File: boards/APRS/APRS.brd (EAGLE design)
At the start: 50.8 x 38.1 mm, 15 parts

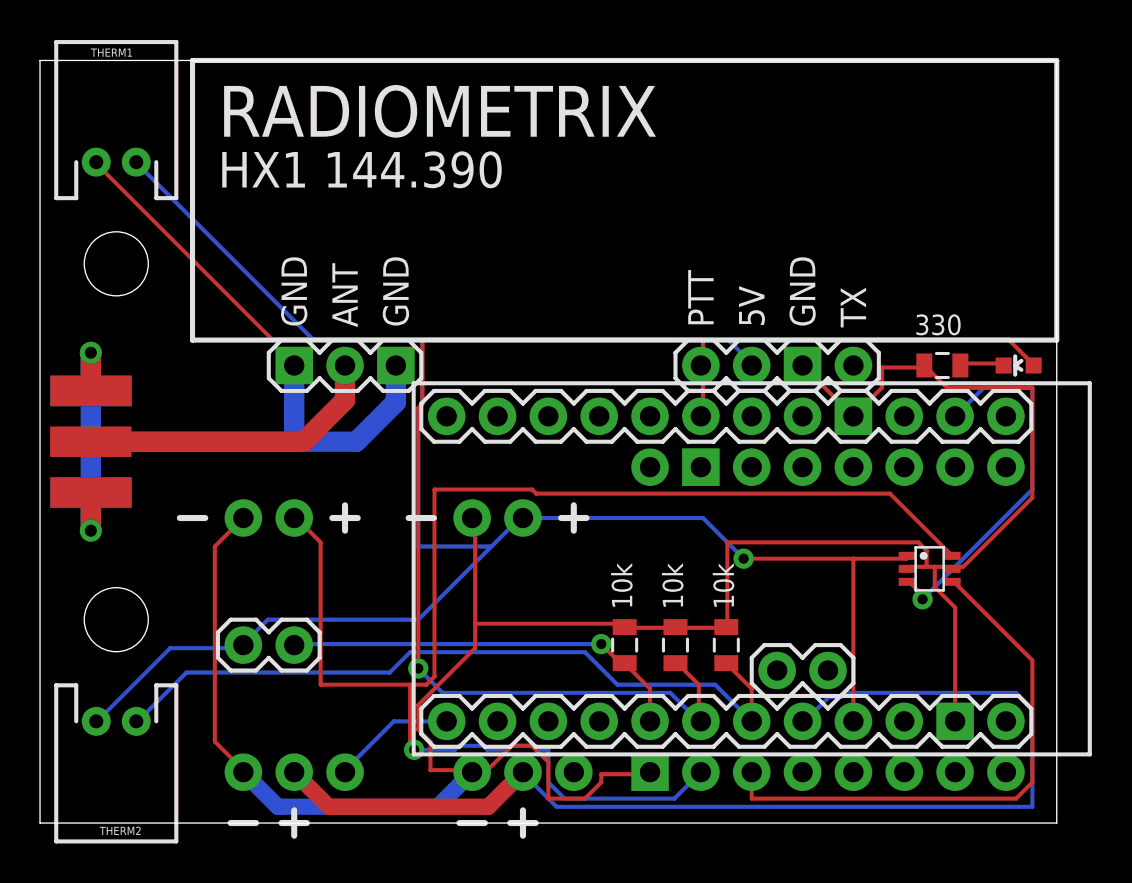
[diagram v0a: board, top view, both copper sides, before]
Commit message: New APRS board, close to ready
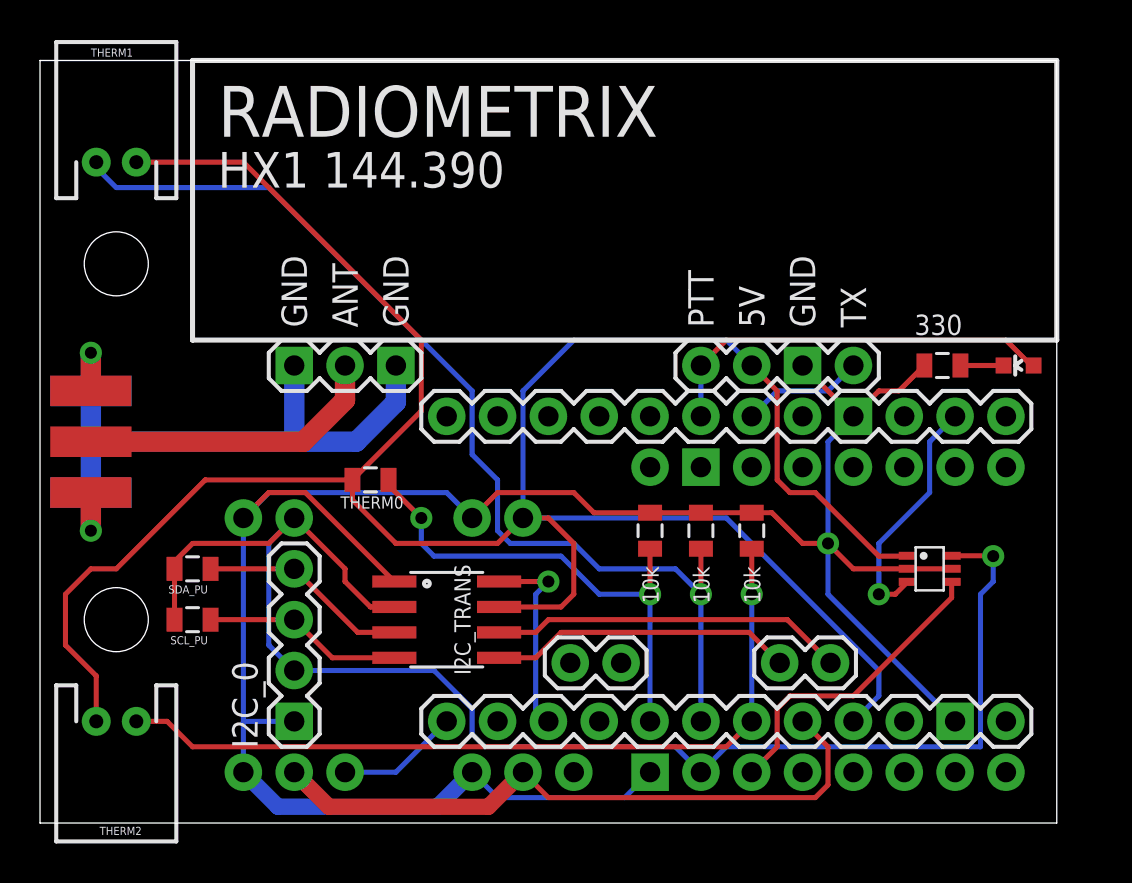
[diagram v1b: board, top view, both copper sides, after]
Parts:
- added I2C_0: (no value), SparkFun-Connectors:1X04
- added I2C_TRANS: PCA9306-D, OpenSpace:SO8
- added SCL_PU, SDA_PU: 3.3k, SparkFun-Passives:0805
- ARDUINO: value ARDUINO_PRO_MINI -> ARDUINO_PRO_MINI-NOSILK; device OpenSpace:ARDUINO_PRO_MINI -> OpenSpace:ARDUINO_PRO_MINI-NOSILK
- GPS0: value VENUS_GPS -> VENUS_GPS-NOSILK; device OpenSpace:VENUS_GPS -> OpenSpace:VENUS_GPS-NOSILK
- POWER3, POWER5: device OpenSpace:POWER-TPS6300X -> OpenSpace:POWER-TPS6300X-NOSILK
- THERM0: value (none) -> 10k; device SparkFun:1X02 -> SparkFun-Passives:0805
- THERM1, THERM2: value (none) -> 10k
- moved THERM0 9.09 mm to (16.5, 17.1), turned to 0 degrees
- moved R_T0 5.85 mm to (30.5, 14.6)
- moved R_T1 5.85 mm to (33.0, 14.6)
- moved R_T2 5.85 mm to (35.6, 14.6)
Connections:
- new net N$4: ARDUINO.A4_SDA, I2C_TRANS.5
- new net N$5: ARDUINO.A5_SCL, I2C_TRANS.6
- new net N$6: ARDUINO.D12, I2C_TRANS.8
- new net SCL: I2C_0.4, I2C_TRANS.3, SDA_PU.1
- new net SDA: I2C_0.3, I2C_TRANS.4, SCL_PU.1
- net 3.3V: now also I2C_0.2, I2C_TRANS.2, SCL_PU.2, SDA_PU.2
- net 5V: now also I2C_TRANS.7, THERM0.1; no longer THERM0.2
- net A0: now also THERM0.2; no longer THERM0.1
- net GND: now also I2C_0.1, I2C_TRANS.1
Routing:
- net 5V: track 103.1 -> 128.3 mm, vias 1 -> 0
- net 1.8V: track 56.3 -> 32.6 mm
- net N$5: track 0.00 -> 17.7 mm
- net N$4: track 0.00 -> 15.2 mm
- net N$3: track 27.4 -> 15.5 mm
- net SCL: track 0.00 -> 10.5 mm
- net N$6: track 0.00 -> 9.97 mm, vias 0 -> 1
- net SDA: track 0.00 -> 9.97 mm
- net RX: track 18.5 -> 12.2 mm
- net GND: track 119.4 -> 113.1 mm, vias 0 -> 1
- net D3: track 0.00 -> 6.13 mm
- net A0: track 20.4 -> 25.0 mm, vias 1 -> 2
- net A1: track 55.3 -> 51.3 mm
- net A2: track 37.0 -> 40.4 mm, vias 0 -> 1
- net 3.3V: track 71.9 -> 75.2 mm
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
